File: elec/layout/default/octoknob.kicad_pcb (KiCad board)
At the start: 2 copper layers, 225.7 x 100.8 mm, 0 parts

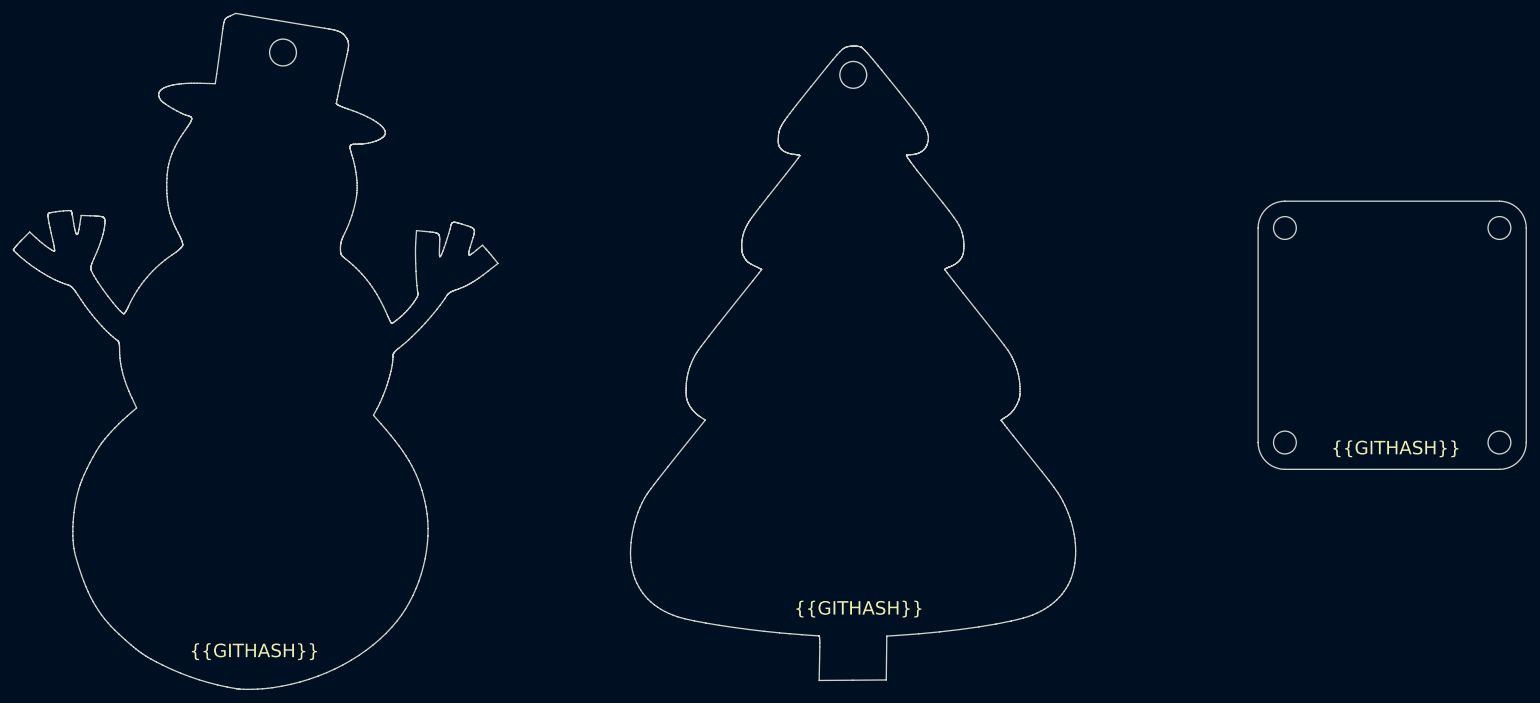
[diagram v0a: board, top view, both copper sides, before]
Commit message: init
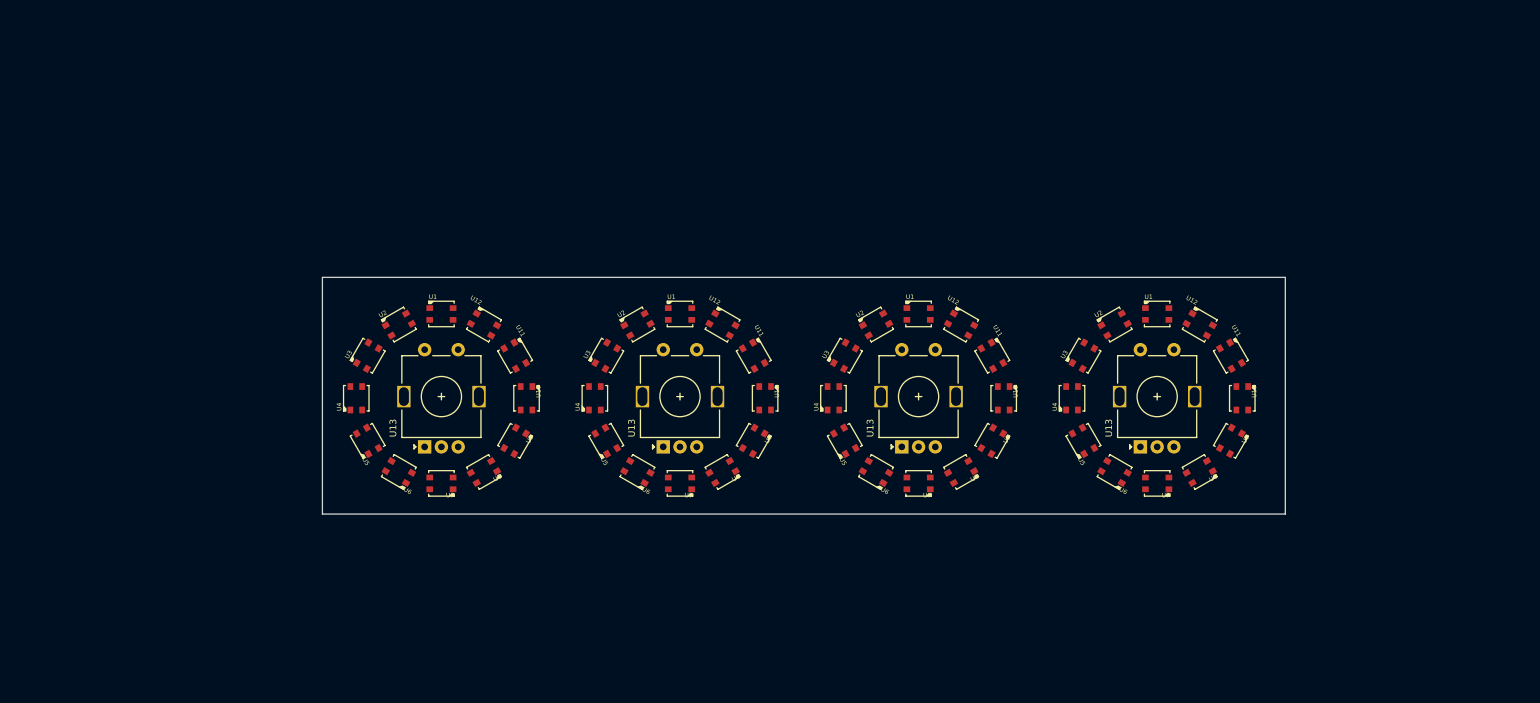
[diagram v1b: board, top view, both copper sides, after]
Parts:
- added U1: , adafruit:LED3535, F.Cu at (99.8, 94.6)
- added U1: , adafruit:LED3535, F.Cu at (206.6, 94.6)
- added U1: , adafruit:LED3535, F.Cu at (171.0, 94.6)
- added U1: , adafruit:LED3535, F.Cu at (135.4, 94.6)
- added U10: , adafruit:LED3535, F.Cu at (112.5, 107.2)
- added U10: , adafruit:LED3535, F.Cu at (148.1, 107.2)
- added U10: , adafruit:LED3535, F.Cu at (183.7, 107.2)
- added U10: , adafruit:LED3535, F.Cu at (219.3, 107.2)
- added U11: , adafruit:LED3535, F.Cu at (217.6, 100.8)
- added U11: , adafruit:LED3535, F.Cu at (146.4, 100.8)
- added U11: , adafruit:LED3535, F.Cu at (110.8, 100.8)
- added U11: , adafruit:LED3535, F.Cu at (182.0, 100.8)
- added U12: , adafruit:LED3535, F.Cu at (106.1, 96.2)
- added U12: , adafruit:LED3535, F.Cu at (212.9, 96.2)
- added U12: , adafruit:LED3535, F.Cu at (177.3, 96.2)
- added U12: , adafruit:LED3535, F.Cu at (141.7, 96.2)
- added U13: , Rotary_Encoder:RotaryEncoder_Alps_EC11E-Switch_Vertical_H20mm, F.Cu at (204.1, 114.4)
- added U13: , Rotary_Encoder:RotaryEncoder_Alps_EC11E-Switch_Vertical_H20mm, F.Cu at (132.9, 114.4)
- added U13: , Rotary_Encoder:RotaryEncoder_Alps_EC11E-Switch_Vertical_H20mm, F.Cu at (168.5, 114.4)
- added U13: , Rotary_Encoder:RotaryEncoder_Alps_EC11E-Switch_Vertical_H20mm, F.Cu at (97.3, 114.4)
- added U2: , adafruit:LED3535, F.Cu at (93.4, 96.2)
- added U2: , adafruit:LED3535, F.Cu at (129.0, 96.2)
- added U2: , adafruit:LED3535, F.Cu at (200.2, 96.2)
- added U2: , adafruit:LED3535, F.Cu at (164.6, 96.2)
- added U3: , adafruit:LED3535, F.Cu at (160.0, 100.8)
- added U3: , adafruit:LED3535, F.Cu at (195.6, 100.8)
- added U3: , adafruit:LED3535, F.Cu at (88.8, 100.8)
- added U3: , adafruit:LED3535, F.Cu at (124.4, 100.8)
- added U4: , adafruit:LED3535, F.Cu at (193.9, 107.2)
- added U4: , adafruit:LED3535, F.Cu at (158.3, 107.2)
- added U4: , adafruit:LED3535, F.Cu at (87.1, 107.2)
- added U4: , adafruit:LED3535, F.Cu at (122.7, 107.2)
- added U5: , adafruit:LED3535, F.Cu at (160.0, 113.5)
- added U5: , adafruit:LED3535, F.Cu at (88.8, 113.5)
- added U5: , adafruit:LED3535, F.Cu at (195.6, 113.5)
- added U5: , adafruit:LED3535, F.Cu at (124.4, 113.5)
- added U6: , adafruit:LED3535, F.Cu at (164.6, 118.2)
- added U6: , adafruit:LED3535, F.Cu at (93.4, 118.2)
- added U6: , adafruit:LED3535, F.Cu at (200.2, 118.2)
- added U6: , adafruit:LED3535, F.Cu at (129.0, 118.2)
- added U7: , adafruit:LED3535, F.Cu at (171.0, 119.9)
- added U7: , adafruit:LED3535, F.Cu at (99.8, 119.9)
- added U7: , adafruit:LED3535, F.Cu at (135.4, 119.9)
- added U7: , adafruit:LED3535, F.Cu at (206.6, 119.9)
- added U8: , adafruit:LED3535, F.Cu at (141.7, 118.2)
- added U8: , adafruit:LED3535, F.Cu at (212.9, 118.2)
- added U8: , adafruit:LED3535, F.Cu at (106.1, 118.2)
- added U8: , adafruit:LED3535, F.Cu at (177.3, 118.2)
- added U9: , adafruit:LED3535, F.Cu at (182.0, 113.5)
- added U9: , adafruit:LED3535, F.Cu at (110.8, 113.5)
- added U9: , adafruit:LED3535, F.Cu at (146.4, 113.5)
- added U9: , adafruit:LED3535, F.Cu at (217.6, 113.5)
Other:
- board size 225.7 x 100.8 mm -> 143.6 x 35.3 mm
- board text removed: "{{GITHASH}}"
